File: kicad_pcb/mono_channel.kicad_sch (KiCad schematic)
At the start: 106 parts, among them IC1 OPA1679, IC2 NE5532, IC4 NE5532, J10 Conn_01x02, J11 Conn_01x02, J2 Conn_01x05, J4 Conn_01x02, J6 Conn_01x03, J8 Conn_01x05

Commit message: modifiche sostanziali al path
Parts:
- removed J11: Conn_01x02, symbol Connector_Generic:Conn_01x02
- removed R89: 75R, 0_Resistors:0603, symbol 0_Basics:R
- added DIR/PROC-CH1, OUT-PRE/POST-CH1: (no value), 0_Switches:SWITCH_PUSH_7X7-POLARIZED, symbol 0_ED-Sounds:SWITCH-PUSH-LATCHING
- added LED-OUT-DIR-CH1, LED-OUT-DIR-CH2, LED-OUT-PROC-CH1, LED-OUT-PROC-CH2: orange, 0_Leds:LED3MM, symbol 0_Basics:LED
- added R100, R101, R98, R99: R, 0_Resistors:0603, symbol 0_Basics:R
- added R102, R96, R97: 75R, 0_Resistors:0603, symbol 0_Basics:R
- added R94, R95: (no value), 0_Resistors:0603, symbol 0_Basics:R
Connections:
- net +5VD is gone; now on net VD: HPF-CH1.2-C (C), INSERT-CH1.2-C (C), J4.1 (Pin_1), PFL-CH1.2-C (C)
- net GND: now also RELAY-2.3, RELAY-3.2, RELAY-3.7, R96.1; no longer J10.2 (Pin_2)
- net GNDD: now also DIR/PROC-CH1.1-NC (NC), R100.2, R101.2, R98.2, R99.2
- net at C25.2, R9.1: now also RELAY-4.5
- net at C39.1, HPF-CH1.1-NC (NC): now also RELAY-4.6
- net at INSERT-CH1.1-C (C), R27.1: now also RELAY-2.6, R97.2
- net at C58.2, IC4.1, R38.1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: now also R94.2
- net at AUX1-CH1.3 (CW), AUX2-CH1.3 (CW), AUX3-CH1.3 (CW)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: now also RELAY-2.4, RELAY-2.7
- net at AUX1-CH1.6 (CW), AUX2-CH1.6 (CW), AUX3-CH1.6 (CW)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: now also R102.2
- net at RELAY-3.3: now also R95.1
- net BUS-AFL-RIGHT: now reaches RELAY-3.4
- net BUS-AFL-LEFT: now reaches RELAY-3.5
- net at RELAY-3.6: now also R94.1
- net at LED-MONITOR-B-CH1.2 (A): now also RELAY-4.2
- net VD: now reaches RELAY-4.3
- net VD: now also DIR/PROC-CH1.1-NO (NO), DIR/PROC-CH1.2-C (C), OUT-PRE/POST-CH1.2-C (C)
- net at RELAY-4.4: now also LED-MONITOR-A-CH1.2 (A)
- net at RELAY-4.7: now also C26.2, R16.1
- net at J10.1 (Pin_1): now also R96.2
- net at C59.2, IC4.7, R39.1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: now also R95.2
- new net: LED-OUT-PROC-CH1.1 (K), R98.1
- new net: J10.2 (Pin_2), OUT-PRE/POST-CH1.1-C (C)
- new net: OUT-PRE/POST-CH1.1-NC (NC), R97.1
- new net: OUT-PRE/POST-CH1.1-NO (NO), R102.1
- new net: LED-OUT-PROC-CH2.1 (K), R101.1
- new net: LED-OUT-DIR-CH1.1 (K), R99.1
- new net: DIR/PROC-CH1.2-NC (NC), LED-OUT-DIR-CH1.2 (A)
- new net: DIR/PROC-CH1.2-NO (NO), LED-OUT-PROC-CH1.2 (A)
- new net: LED-OUT-PROC-CH2.2 (A), OUT-PRE/POST-CH1.2-NO (NO)
- new net: LED-OUT-DIR-CH2.1 (K), R100.1
- new net: LED-OUT-DIR-CH2.2 (A), OUT-PRE/POST-CH1.2-NC (NC)
- no-connect marks 3 -> 5
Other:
- note added: "bisognerebbe fare mirror del postfader"
- note added: "collegare"
- note removed: "CAPIRE COME"
- note removed: "afl con relay"
- note removed: "capire se unico connettore"
- note removed: "coppia di opamp che isola"
- note removed: "dopo il routing valutare se posso metterne altre in parallelo"
- note removed: "metering in routing capire se meglio unico connettore da 6 o 8"
- note removed: "postfade output stereo oppure mono prima del pan"
- moved on the sheet: AUX1-CH1A, AUX1-CH1B, AUX2-CH1A, AUX2-CH1B, AUX3-CH1A, AUX3-CH1B, AUX4-CH1A, AUX4-CH1B, C25, C26, C27, C34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

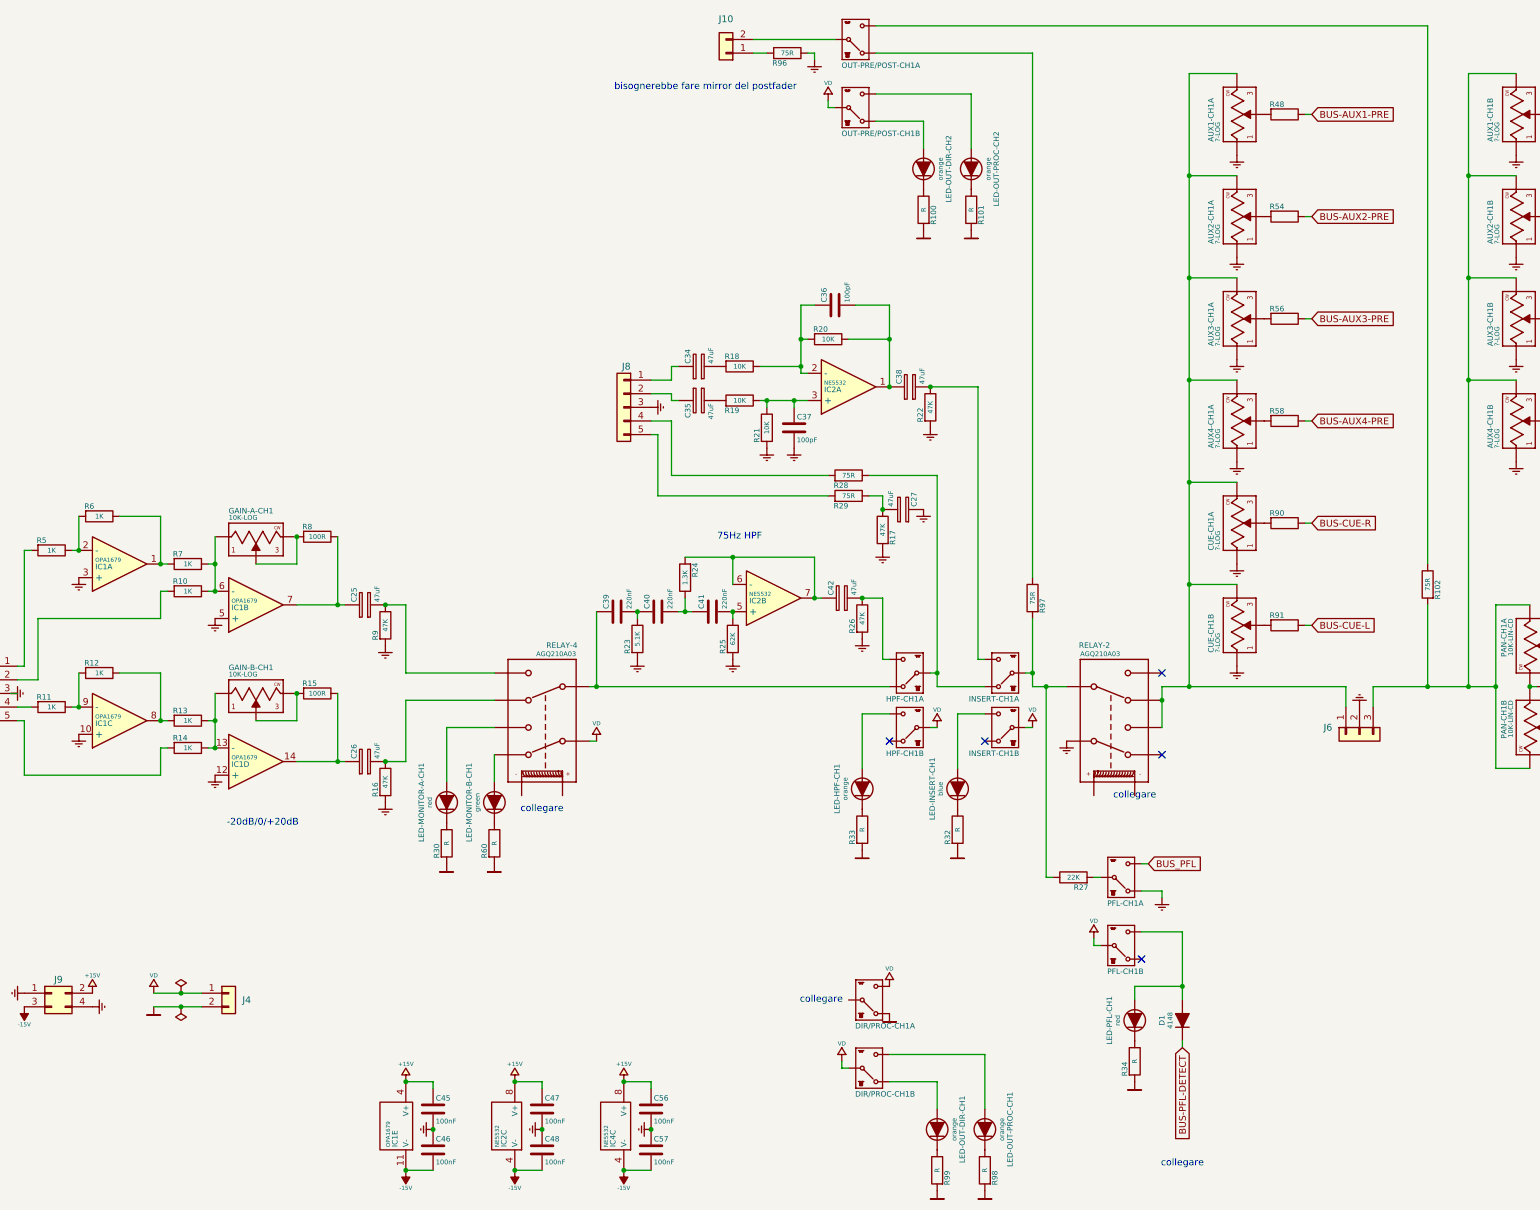
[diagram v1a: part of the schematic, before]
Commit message: altre cose
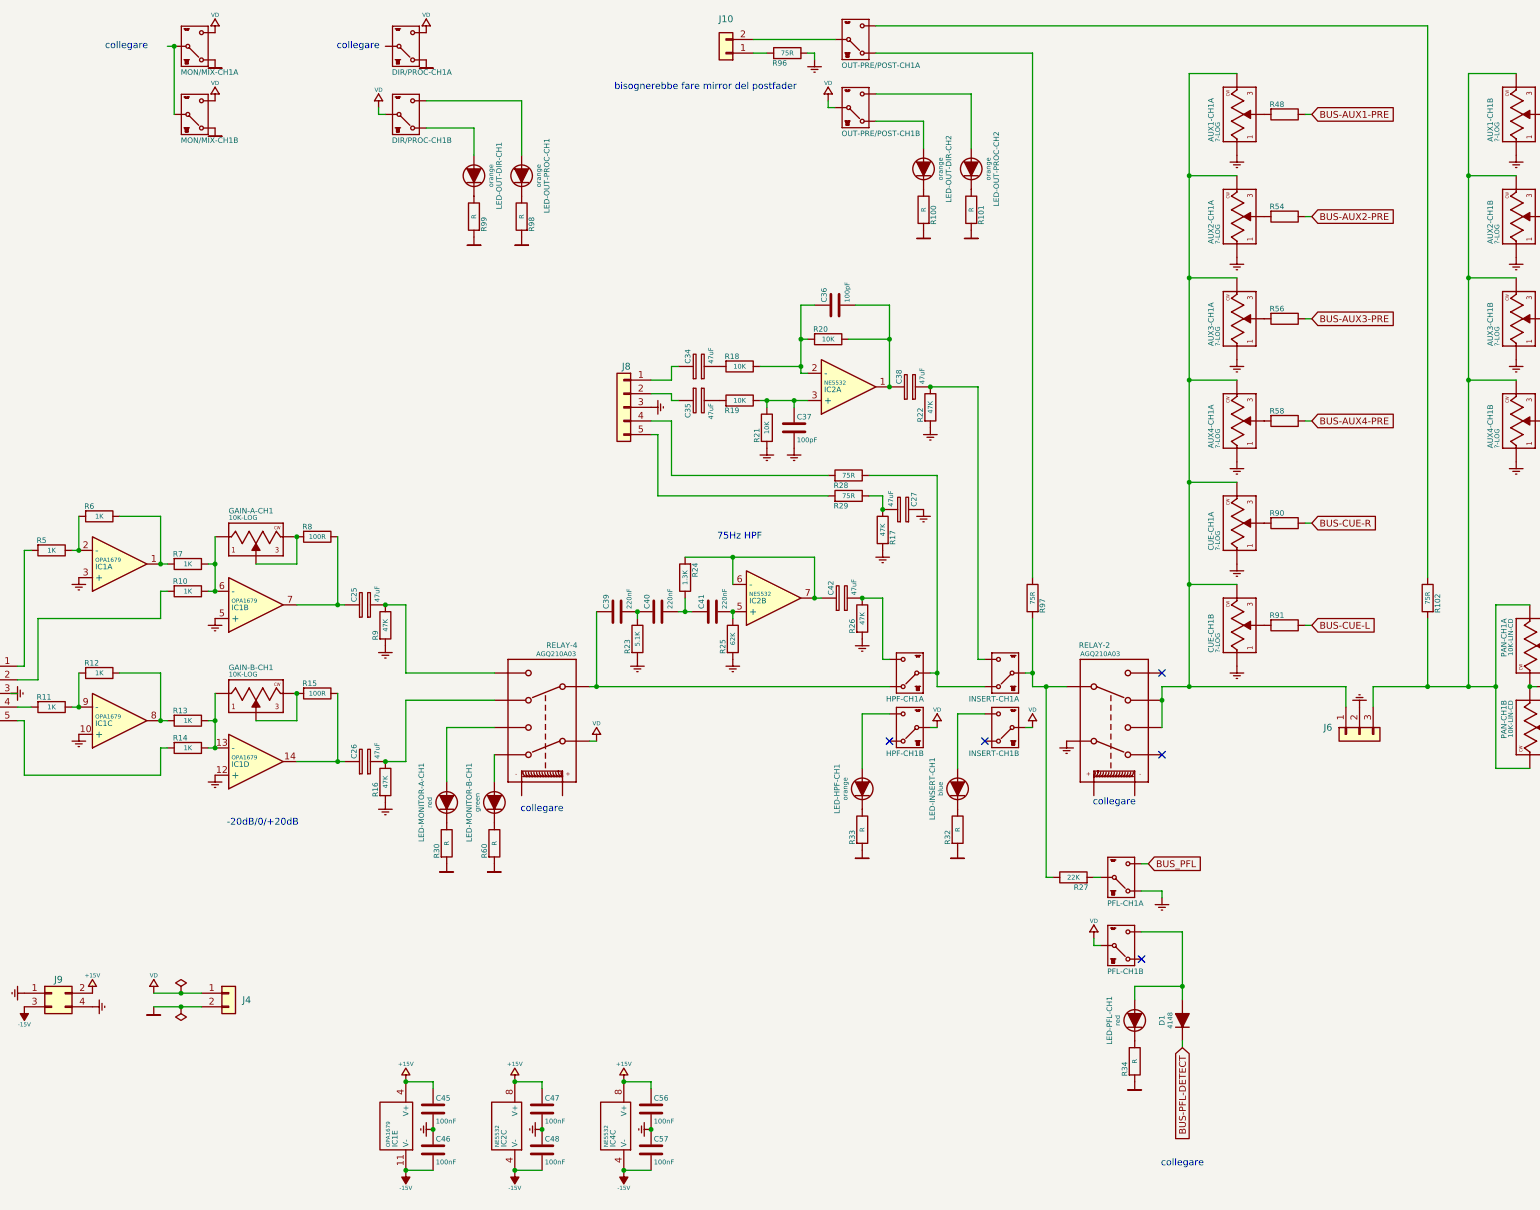
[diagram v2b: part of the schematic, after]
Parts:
- added MON/MIX-CH1: (no value), 0_Switches:SWITCH_PUSH_7X7-POLARIZED, symbol 0_ED-Sounds:SWITCH-PUSH-LATCHING
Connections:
- net GNDD: now also MON/MIX-CH1.1-NC (NC), MON/MIX-CH1.2-NC (NC)
- net VD: now also MON/MIX-CH1.1-NO (NO), MON/MIX-CH1.2-NO (NO)
- new net: MON/MIX-CH1.1-C (C), MON/MIX-CH1.2-C (C)
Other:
- moved on the sheet: DIR/PROC-CH1A, DIR/PROC-CH1B, LED-OUT-DIR-CH1, LED-OUT-PROC-CH1, R102, R98, R99

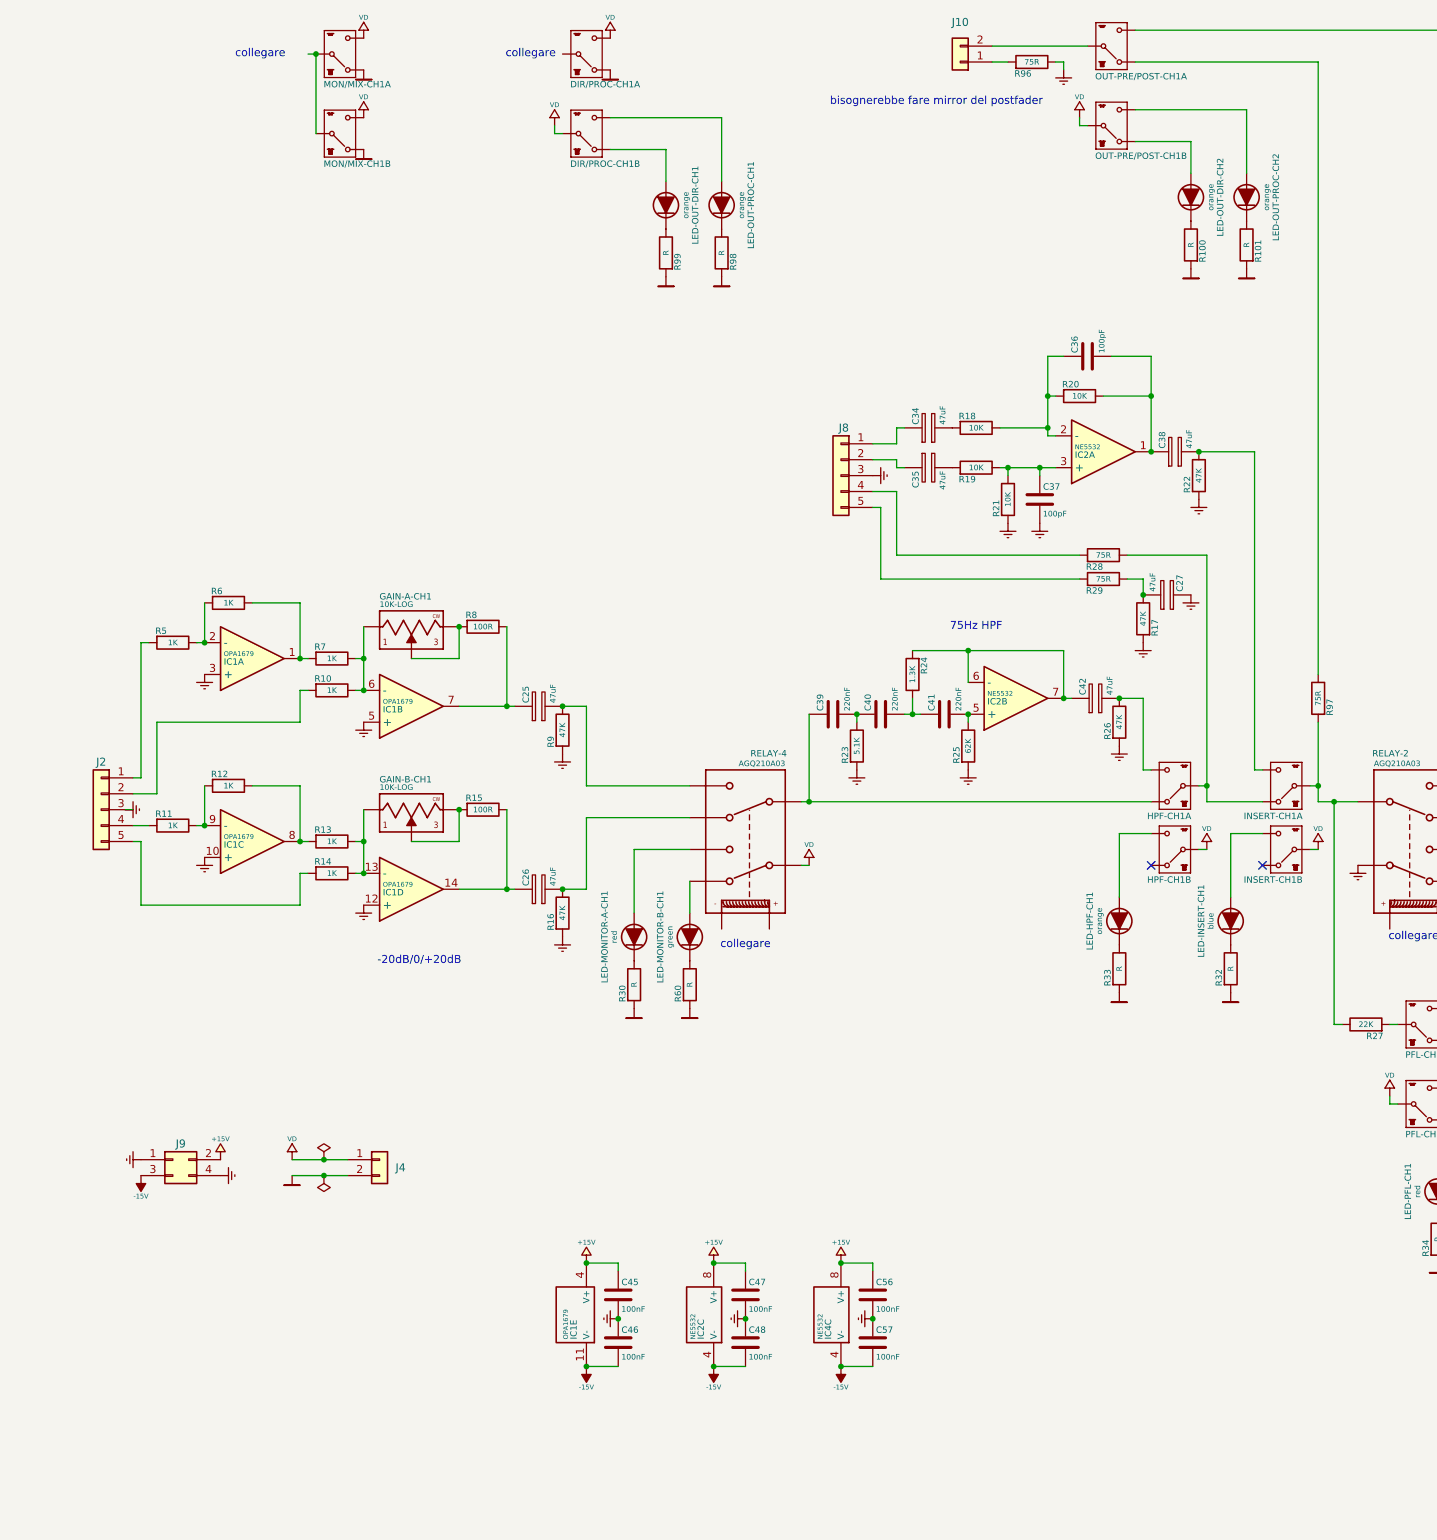
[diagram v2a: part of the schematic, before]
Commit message: fx bypass
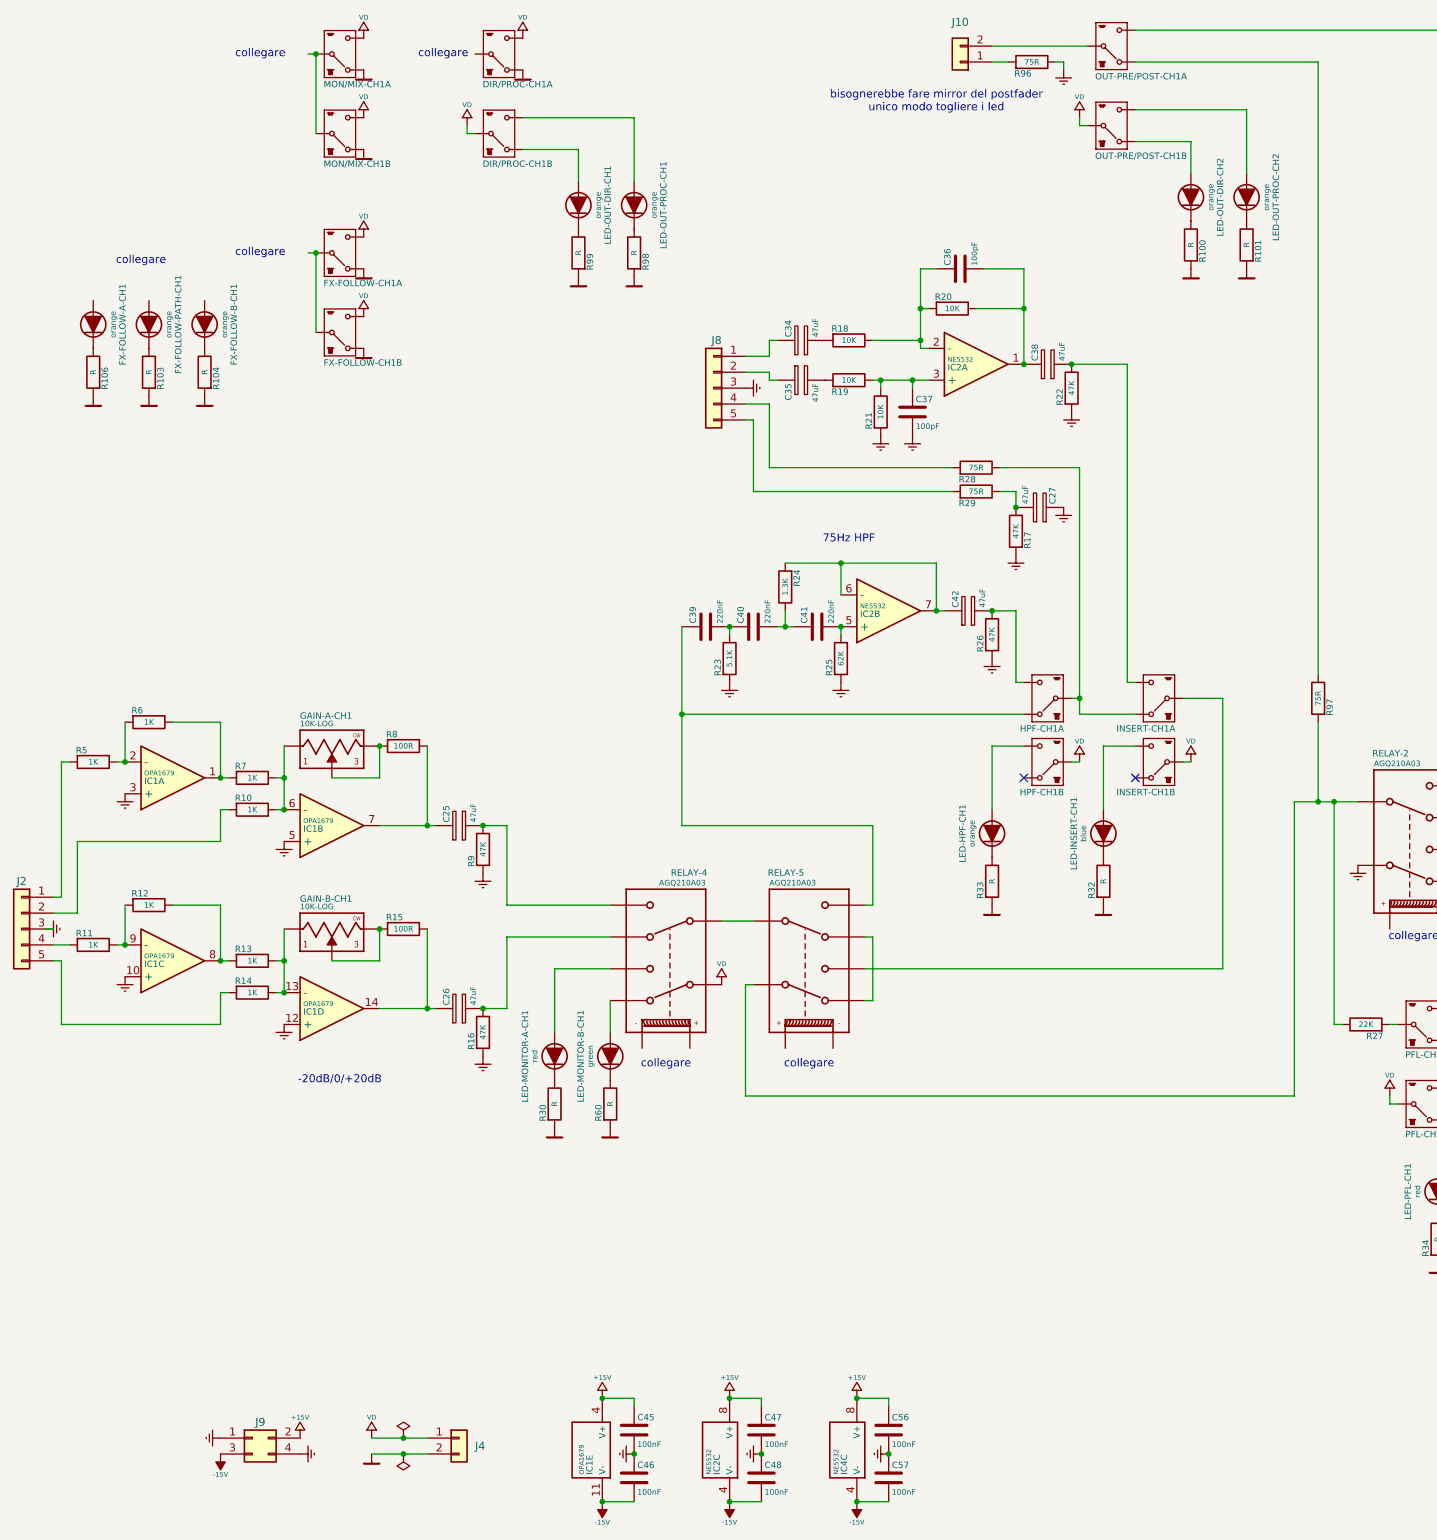
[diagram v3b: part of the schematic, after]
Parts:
- added FX-FOLLOW-A-CH1, FX-FOLLOW-B-CH1, FX-FOLLOW-PATH-CH1: orange, 0_Leds:LED3MM, symbol 0_Basics:LED
- added FX-FOLLOW-CH1: (no value), 0_Switches:SWITCH_PUSH_7X7-POLARIZED, symbol 0_ED-Sounds:SWITCH-PUSH-LATCHING
- added R103, R104, R106: R, 0_Resistors:0603, symbol 0_Basics:R
- added RELAY-5: AGQ210A03, 0_Switches:FTRB3GA45ZB10, symbol 0_ED-Sounds:RELAY_AGQ210
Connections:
- net GNDD: now also FX-FOLLOW-CH1.1-NC (NC), FX-FOLLOW-CH1.2-NC (NC), R103.2, R104.2, R106.2
- net VD: now also FX-FOLLOW-CH1.1-NO (NO), FX-FOLLOW-CH1.2-NO (NO)
- net at C39.1, HPF-CH1.1-NC (NC): now also RELAY-5.5; no longer RELAY-4.6
- net at R27.1, R97.2, RELAY-2.6: now also RELAY-5.3; no longer INSERT-CH1.1-C (C)
- new net: FX-FOLLOW-CH1.1-C (C), FX-FOLLOW-CH1.2-C (C)
- new net: FX-FOLLOW-A-CH1.1 (K), R106.1
- new net: RELAY-4.6, RELAY-5.6
- new net: INSERT-CH1.1-C (C), RELAY-5.4
- new net: FX-FOLLOW-B-CH1.1 (K), R104.1
- new net: FX-FOLLOW-PATH-CH1.1 (K), R103.1
- new net: RELAY-5.2, RELAY-5.7
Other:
- note added: "bisognerebbe fare mirror del postfader unico modo togliere i led"
- note removed: "bisognerebbe fare mirror del postfader"
- moved on the sheet: C25, C26, C27, C34, C35, C36, C37, C38, C39, C40, C41, C42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
